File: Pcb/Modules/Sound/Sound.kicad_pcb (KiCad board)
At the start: 2 copper layers, 50.8 x 20.3 mm, 18 parts, among them J1 JACK_RJ45, U1 MAX4466, X1 HOLE, X2 HOLE, X3 HOLE, X4 HOLE

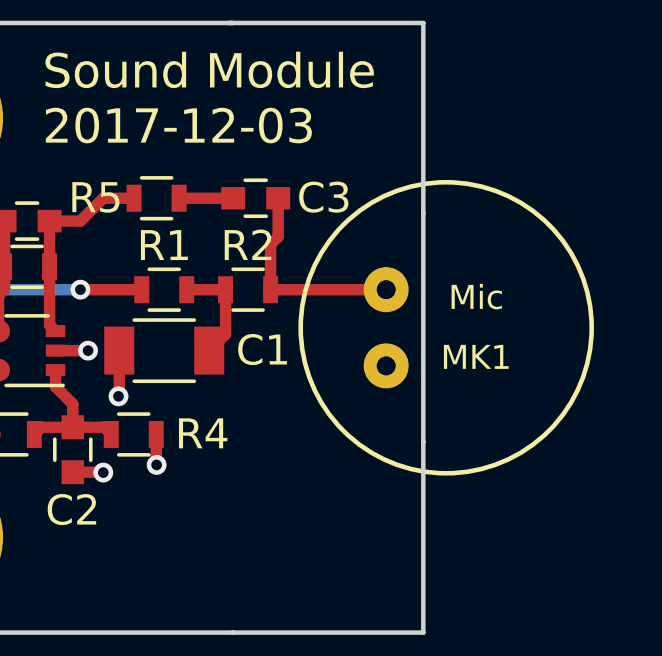
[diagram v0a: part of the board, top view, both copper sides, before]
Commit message: Update pcbs.
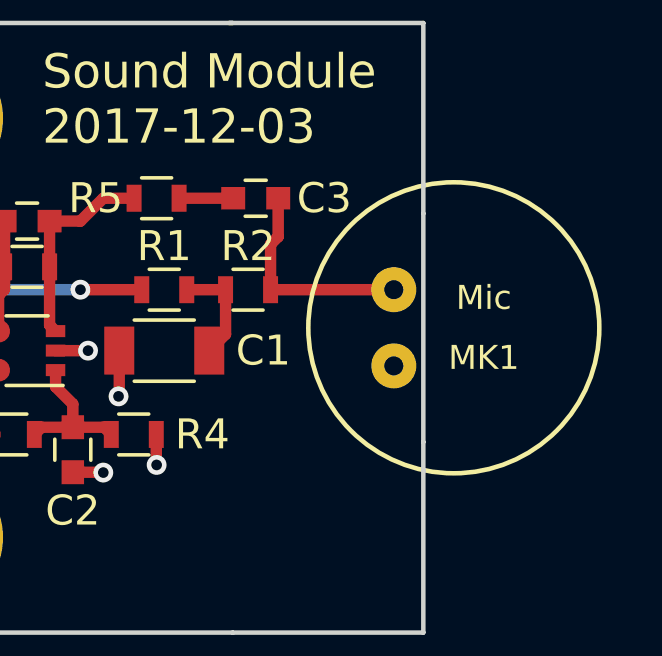
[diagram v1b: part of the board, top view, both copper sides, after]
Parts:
- moved MK1 0.25 mm to (77.2, 35.6)
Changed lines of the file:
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@@
   )
   (setup
-    (last_trace_width 0.381)
+    (last_trace_width 0.254)
     (user_trace_width 0.381)
     (user_trace_width 0.508)
@@
   )
   (module CA6:MIC_CMA-4544PF (layer F.Cu)
-    (at 76.962 35.56 180)
+    (at 77.216 35.56 180)
     (tags "CMS SM")
     (attr smd)
